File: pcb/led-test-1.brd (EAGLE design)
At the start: 17.8 x 14.6 mm, 2 parts

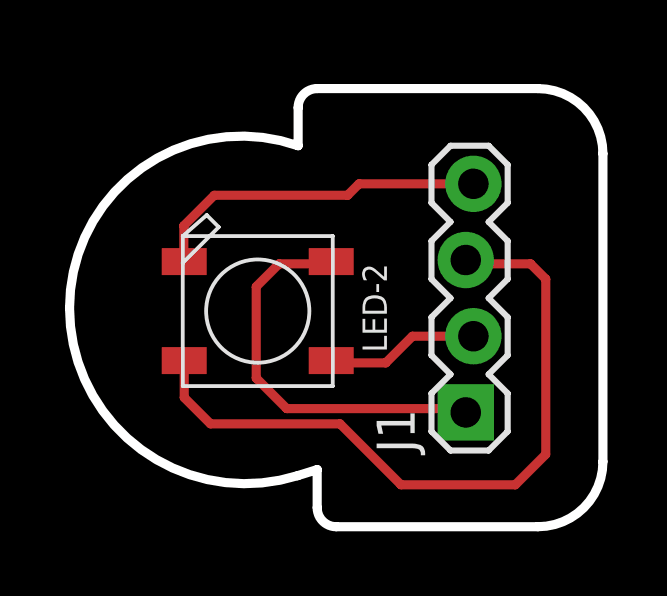
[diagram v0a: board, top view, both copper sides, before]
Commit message: added led-test v2
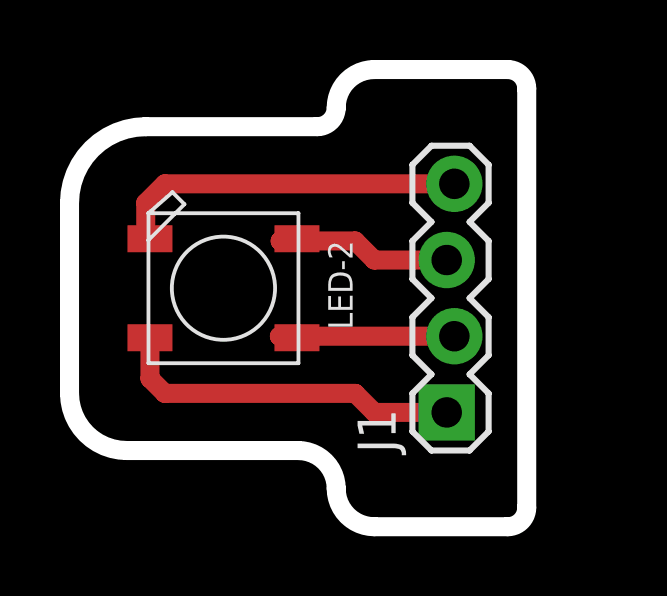
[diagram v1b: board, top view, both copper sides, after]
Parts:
- moved LED-2 1.37 mm to (24.8, 40.3)
- moved J1 0.64 mm to (32.4, 36.2)
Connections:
- removed net N$2 (its old number): J1.1, LED-2.2-DOUT
- removed net N$4 (its old number): J1.3, LED-2.4-DIN
- new net N$1: J1.1, LED-2.4-DIN
- new net N$3: J1.3, LED-2.2-DOUT
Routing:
- net N$4 (its old number): track 23.7 -> 0.00 mm
- net N$2 (its old number): track 13.4 -> 0.00 mm
- net N$1: track 0.00 -> 11.7 mm
- net N$3: track 0.00 -> 6.38 mm
- net N$2: track 5.14 -> 6.42 mm
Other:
- board size 17.8 x 14.6 mm -> 15.2 x 15.2 mm
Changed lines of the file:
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@@
 <setting verticaltext="up"/>
 </settings>
-<grid distance="10" unitdist="mil" unit="mil" style="dots" multiple="1" display="yes" altdistance="10" altunitdist="mil" altunit="mil"/>
+<grid distance="25" unitdist="mil" unit="mil" style="dots" multiple="1" display="yes" altdistance="10" altunitdist="mil" altunit="mil"/>
 <layers>
 <layer number="1" name="Top" color="4" fill="1" visible="yes" active="yes"/>
@@
 <board>
 <plain>
-<wire x1="27.94" y1="34.29" x2="27.2905125" y2="34.086734375" width="0.3048" layer="20"/>
-<wire x1="27.2905125" y1="34.086734375" x2="19.685" y2="39.675765625" width="0.3048" layer="20" curve="-107.378173"/>
-<wire x1="19.685" y1="39.675765625" x2="27.305" y2="45.085" width="0.3048" layer="20" curve="-109.260162"/>
-<wire x1="27.305" y1="45.085" x2="27.305" y2="46.355" width="0.3048" layer="20"/>
-<wire x1="27.305" y1="46.355" x2="27.94" y2="46.99" width="0.3048" layer="20" curve="-90"/>
-<wire x1="27.94" y1="46.99" x2="35.296978125" y2="46.99" width="0.3048" layer="20"/>
-<wire x1="35.296978125" y1="46.99" x2="37.465" y2="44.821978125" width="0.3048" layer="20" curve="-90"/>
-<wire x1="37.465" y1="44.821978125" x2="37.465" y2="34.553021875" width="0.3048" layer="20"/>
-<wire x1="37.465" y1="34.553021875" x2="35.296978125" y2="32.385" width="0.3048" layer="20" curve="-90"/>
-<wire x1="35.296978125" y1="32.385" x2="28.575" y2="32.385" width="0.3048" layer="20"/>
-<wire x1="28.575" y1="32.385" x2="27.94" y2="33.02" width="0.3048" layer="20" curve="-90"/>
-<wire x1="27.94" y1="33.02" x2="27.94" y2="34.29" width="0.3048" layer="20"/>
+<wire x1="34.925" y1="46.99" x2="34.925" y2="33.02" width="0.635" layer="20"/>
+<wire x1="34.925" y1="46.99" x2="34.29" y2="47.625" width="0.635" layer="20" curve="90"/>
+<wire x1="34.29" y1="47.625" x2="29.845" y2="47.625" width="0.635" layer="20"/>
+<wire x1="29.845" y1="47.625" x2="28.575" y2="46.355" width="0.635" layer="20" curve="90"/>
+<wire x1="28.575" y1="46.355" x2="27.94" y2="45.72" width="0.635" layer="20" curve="-90"/>
+<wire x1="27.94" y1="45.72" x2="22.225" y2="45.72" width="0.635" layer="20"/>
+<wire x1="22.225" y1="45.72" x2="19.685" y2="43.18" width="0.635" layer="20" curve="90"/>
+<wire x1="19.685" y1="43.18" x2="19.685" y2="36.83" width="0.635" layer="20"/>
+<wire x1="34.925" y1="33.02" x2="34.29" y2="32.385" width="0.635" layer="20" curve="-90"/>
+<wire x1="34.29" y1="32.385" x2="29.845" y2="32.385" width="0.635" layer="20"/>
+<wire x1="29.845" y1="32.385" x2="28.575" y2="33.655" width="0.635" layer="20" curve="-90"/>
+<wire x1="28.575" y1="33.655" x2="27.305" y2="34.925" width="0.635" layer="20" curve="90"/>
+<wire x1="27.305" y1="34.925" x2="21.59" y2="34.925" width="0.635" layer="20"/>
+<wire x1="21.59" y1="34.925" x2="19.685" y2="36.83" width="0.635" layer="20" curve="-90"/>
 </plain>
 <attributes>
@@
 </autorouter>
 <elements>
-<element name="LED-2" library="adafruit" library_urn="urn:adsk.eagle:library:420" package="WS2812B" value="WS2812B5050" x="25.9588" y="39.5732"/>
-<element name="J1" library="SparkFun-Connectors" package="1X04_LOCK" value="" x="33.02" y="36.195" rot="R90">
-<attribute name="PROD_ID" value="CONN-09696" x="33.02" y="36.195" size="1.778" layer="27" rot="R90" display="off"/>
+<element name="LED-2" library="adafruit" library_urn="urn:adsk.eagle:library:420" package="WS2812B" value="WS2812B5050" x="24.8158" y="40.3352"/>
+<element name="J1" library="SparkFun-Connectors" package="1X04_LOCK" value="" x="32.385" y="36.195" rot="R90">
+<attribute name="PROD_ID" value="CONN-09696" x="32.385" y="36.195" size="1.778" layer="27" rot="R90" display="off"/>
 </element>
 </elements>
 <signals>
 <signal name="N$1">
-<contactref element="LED-2" pad="3-GND"/>
-<contactref element="J1" pad="4"/>
-<wire x1="23.5088" y1="41.2232" x2="23.495" y2="41.237" width="0.3048" layer="1" curve="-90"/>
-<wire x1="23.495" y1="41.237" x2="23.495" y2="42.418" width="0.3048" layer="1"/>
-<wire x1="28.956" y1="43.434" x2="29.337" y2="43.815" width="0.3048" layer="1"/>
-<wire x1="33.147" y1="43.815" x2="29.337" y2="43.815" width="0.3048" layer="1"/>
-<wire x1="23.495" y1="42.418" x2="24.511" y2="43.434" width="0.3048" layer="1"/>
-<wire x1="24.511" y1="43.434" x2="28.956" y2="43.434" width="0.3048" layer="1"/>
+<contactref element="J1" pad="1"/>
+<contactref element="LED-2" pad="4-DIN"/>
+<wire x1="22.86" y1="36.83" x2="22.3658" y2="37.3242" width="0.635" layer="1"/>
+<wire x1="22.3658" y1="38.6852" x2="22.3658" y2="37.3242" width="0.635" layer="1"/>
+<wire x1="29.845" y1="36.195" x2="29.21" y2="36.83" width="0.635" layer="1"/>
+<wire x1="32.258" y1="36.195" x2="29.845" y2="36.195" width="0.635" layer="1"/>
+<wire x1="29.21" y1="36.83" x2="22.86" y2="36.83" width="0.635" layer="1"/>
 </signal>
 <signal name="N$2">
-<contactref element="LED-2" pad="2-DOUT"/>
-<contactref element="J1" pad="1"/>
-<wire x1="25.908" y1="37.338" x2="26.924" y2="36.322" width="0.3048" layer="1"/>
-<wire x1="32.258" y1="36.322" x2="32.385" y2="36.195" width="0.3048" layer="1" curve="90"/>
-<wire x1="32.385" y1="36.195" x2="32.893" y2="36.195" width="0.3048" layer="1"/>
-<wire x1="26.924" y1="36.322" x2="32.258" y2="36.322" width="0.3048" layer="1"/>
-<wire x1="28.4088" y1="41.2232" x2="28.3336" y2="41.148" width="0.3048" layer="1"/>
-<wire x1="28.3336" y1="41.148" x2="26.67" y2="41.148" width="0.3048" layer="1"/>
-<wire x1="26.67" y1="41.148" x2="25.908" y2="40.386" width="0.3048" layer="1"/>
-<wire x1="25.908" y1="40.386" x2="25.908" y2="37.338" width="0.3048" layer="1"/>
+<contactref element="J1" pad="2"/>
+<contactref element="LED-2" pad="1-VDD"/>
+<wire x1="32.512" y1="38.735" x2="26.6806" y2="38.735" width="0.635" layer="1"/>
+<wire x1="26.6806" y1="38.735" x2="27.2658" y2="38.6852" width="0.635" layer="1"/>
 </signal>
 <signal name="N$3">
-<contactref element="LED-2" pad="1-VDD"/>
-<contactref element="J1" pad="2"/>
-<wire x1="28.4088" y1="37.9232" x2="28.486" y2="37.846" width="0.3048" layer="1"/>
-<wire x1="28.486" y1="37.846" x2="30.226" y2="37.846" width="0.3048" layer="1"/>
-<wire x1="30.226" y1="37.846" x2="31.115" y2="38.735" width="0.3048" layer="1"/>
-<wire x1="31.115" y1="38.735" x2="33.147" y2="38.735" width="0.3048" layer="1"/>
+<contactref element="LED-2" pad="2-DOUT"/>
+<contactref element="J1" pad="3"/>
+<wire x1="27.2658" y1="41.9852" x2="26.706" y2="41.91" width="0.635" layer="1"/>
+<wire x1="26.706" y1="41.91" x2="29.21" y2="41.91" width="0.635" layer="1"/>
+<wire x1="29.21" y1="41.91" x2="29.845" y2="41.275" width="0.635" layer="1"/>
+<wire x1="29.845" y1="41.275" x2="32.258" y2="41.275" width="0.635" layer="1"/>
 </signal>
 <signal name="N$4">
-<contactref element="LED-2" pad="4-DIN"/>
-<contactref element="J1" pad="3"/>
-<wire x1="32.893" y1="41.275" x2="33.02" y2="41.148" width="0.3048" layer="1" curve="90"/>
-<wire x1="33.02" y1="41.148" x2="35.052" y2="41.148" width="0.3048" layer="1"/>
-<wire x1="35.052" y1="41.148" x2="35.56" y2="40.64" width="0.3048" layer="1"/>
-<wire x1="34.544" y1="33.782" x2="30.734" y2="33.782" width="0.3048" layer="1"/>
-<wire x1="24.384" y1="35.814" x2="23.5088" y2="36.6892" width="0.3048" layer="1"/>
-<wire x1="23.5088" y1="36.6892" x2="23.5088" y2="37.9232" width="0.3048" layer="1"/>
-<wire x1="35.56" y1="40.64" x2="35.56" y2="34.798" width="0.3048" layer="1"/>
-<wire x1="35.56" y1="34.798" x2="34.544" y2="33.782" width="0.3048" layer="1"/>
-<wire x1="30.734" y1="33.782" x2="28.702" y2="35.814" width="0.3048" layer="1"/>
-<wire x1="28.702" y1="35.814" x2="24.384" y2="35.814" width="0.3048" layer="1"/>
+<contactref element="J1" pad="4"/>
+<contactref element="LED-2" pad="3-GND"/>
+<wire x1="22.3658" y1="41.9852" x2="22.225" y2="42.126" width="0.635" layer="1"/>
+<wire x1="22.225" y1="42.126" x2="22.225" y2="43.18" width="0.635" layer="1"/>
+<wire x1="22.225" y1="43.18" x2="22.86" y2="43.815" width="0.635" layer="1"/>
+<wire x1="22.86" y1="43.815" x2="32.512" y2="43.815" width="0.635" layer="1"/>
 </signal>
 </signals>
